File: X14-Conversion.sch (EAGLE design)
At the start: 23 parts, among them P1 282837-2, P2 282837-2, P3 282837-2

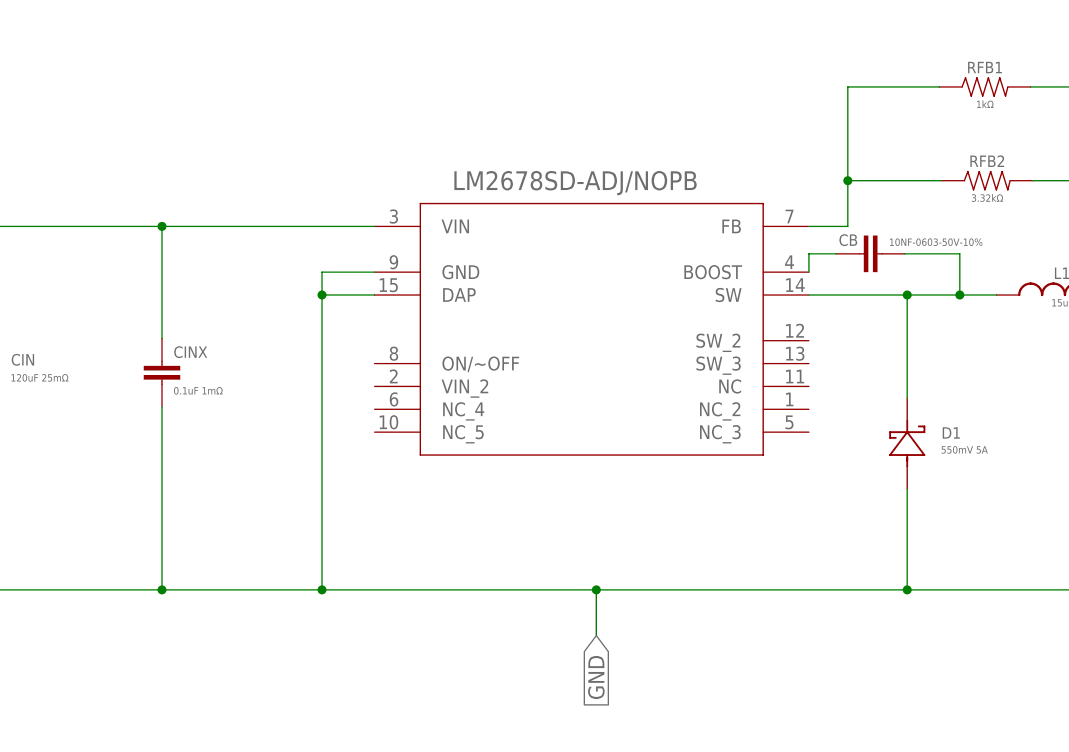
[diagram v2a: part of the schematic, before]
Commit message: Fix Board Layout
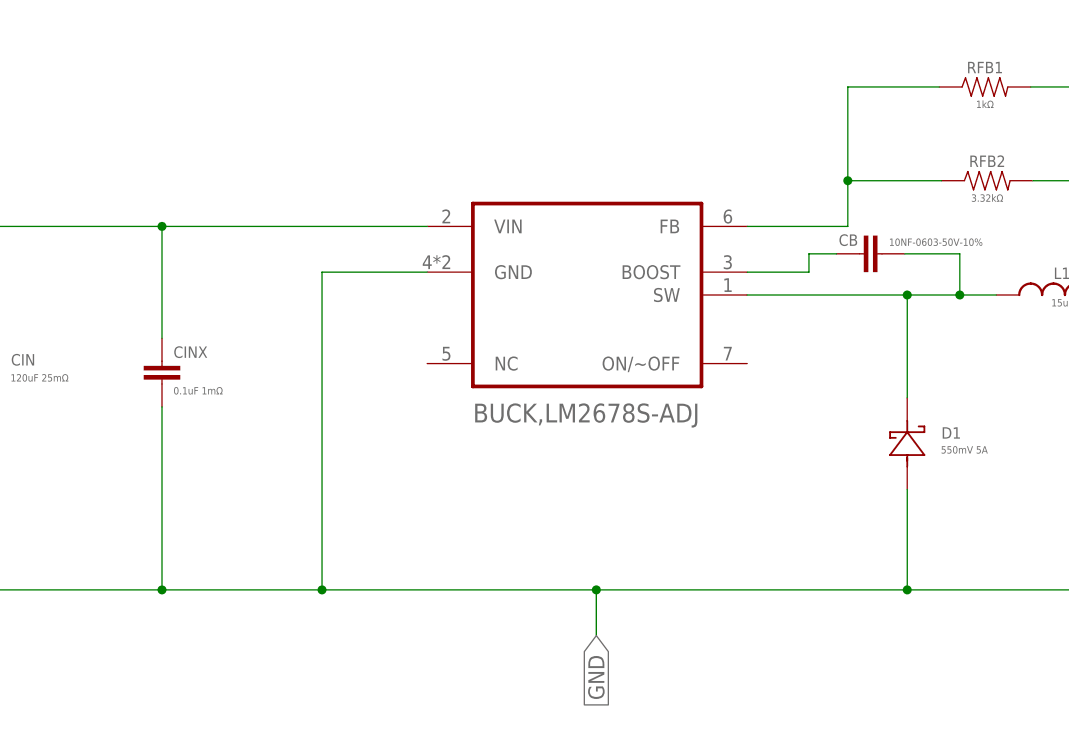
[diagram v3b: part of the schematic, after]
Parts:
- removed LM2678: LM2678SD-ADJ/NOPB, LM2678SX-ADJNOPB:LM2678SD-ADJ/NOPB
- added U1: BUCK,LM2678S-ADJ, BUCK, LM2678S-ADJ:BUCK,LM2678S-ADJ
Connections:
- net 12V: now also U1.VIN; no longer LM2678.VIN
- net GND: now also U1.GND; no longer LM2678.DAP, LM2678.GND
- net N$2: now also U1.SW; no longer LM2678.SW
- net N$4: now also U1.BOOST; no longer LM2678.BOOST
- net N$5: now also U1.FB; no longer LM2678.FB
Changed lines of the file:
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@@
 <part name="FRAME1" library="frames" library_urn="urn:adsk.eagle:library:229" deviceset="A3L-LOC" device=""/>
 <part name="AZ1117C" library="AZ1117C-3.3" deviceset="SOT150P410X160-3N" device="" value="AZ1117C-3.3"/>
-<part name="LM2678" library="LM2678SX-ADJNOPB" deviceset="LM2678SD-ADJ/NOPB" device=""/>
 <part name="U$2" library="testpoints" deviceset="3.3V_TESTPOINT" device=""/>
 <part name="U$3" library="testpoints" deviceset="5.2V_TESTPOINT" device=""/>
@@
 <part name="C3" library="SparkFun-Capacitors" library_urn="urn:adsk.eagle:library:510" deviceset="0.1UF" device="-0603-25V-(+80/-20%)" package3d_urn="urn:adsk.eagle:package:37414/1" value="0.1uF"/>
 <part name="CONN" library="CONN, Distribution-Conversion (3)" deviceset="CONVERSION-DISTRIBUTION" device=""/>
+<part name="U1" library="BUCK, LM2678S-ADJ" deviceset="BUCK,LM2678S-ADJ" device=""/>
 </parts>
 <sheets>
@@
 </instance>
 <instance part="AZ1117C" gate="G$1" x="-75.692" y="-10.668" smashed="yes"/>
-<instance part="LM2678" gate="A" x="-2.54" y="66.04" smashed="yes">
-<attribute name="NAME" x="-13.6144" y="79.9846" size="2.0828" layer="95" ratio="6" rot="SR0" display="off"/>
-<attribute name="VALUE" x="-13.4874" y="77.4446" size="2.0828" layer="96" ratio="6" rot="SR0"/>
-</instance>
 <instance part="U$2" gate="G$1" x="17.78" y="-2.54" smashed="yes"/>
 <instance part="U$3" gate="G$1" x="17.78" y="-12.7" smashed="yes"/>
@@
 <instance part="CONN" gate="G$1" x="-81.28" y="-81.28" smashed="yes">
 <attribute name="NAME" x="-88.9" y="-73.66" size="1.778" layer="95"/>
+</instance>
+<instance part="U1" gate="A" x="1.524" y="65.786" smashed="yes">
+<attribute name="NAME" x="-11.176" y="76.946" size="2.0828" layer="95" ratio="10" rot="SR0" display="off"/>
+<attribute name="VALUE" x="-11.176" y="51.626" size="2.0828" layer="96" ratio="10" rot="SR0"/>
 </instance>
 </instances>
@@
 <wire x1="-45.72" y1="33.02" x2="-27.94" y2="33.02" width="0.1524" layer="91"/>
 <junction x="2.54" y="33.02"/>
-<pinref part="LM2678" gate="A" pin="GND"/>
 <wire x1="-27.94" y1="33.02" x2="2.54" y2="33.02" width="0.1524" layer="91"/>
-<wire x1="-22.098" y1="68.326" x2="-27.94" y2="68.326" width="0.1524" layer="91"/>
-<wire x1="-27.94" y1="68.326" x2="-27.94" y2="65.786" width="0.1524" layer="91"/>
 <junction x="-27.94" y="33.02"/>
-<pinref part="LM2678" gate="A" pin="DAP"/>
-<wire x1="-27.94" y1="65.786" x2="-27.94" y2="33.02" width="0.1524" layer="91"/>
-<wire x1="-22.098" y1="65.786" x2="-27.94" y2="65.786" width="0.1524" layer="91"/>
-<junction x="-27.94" y="65.786"/>
+<wire x1="-27.94" y1="68.326" x2="-27.94" y2="33.02" width="0.1524" layer="91"/>
 <wire x1="-45.72" y1="33.02" x2="-66.04" y2="33.02" width="0.1524" layer="91"/>
 <wire x1="-66.04" y1="33.02" x2="-66.04" y2="53.34" width="0.1524" layer="91"/>
@@
 <pinref part="CIN" gate="G$1" pin="2"/>
 <pinref part="C3" gate="G$1" pin="2"/>
+<pinref part="U1" gate="A" pin="GND"/>
+<wire x1="-27.94" y1="68.326" x2="-16.256" y2="68.326" width="0.1524" layer="91"/>
 </segment>
 <segment>
@@
 <net name="12V" class="0">
 <segment>
-<pinref part="LM2678" gate="A" pin="VIN"/>
-<wire x1="-22.098" y1="73.406" x2="-45.72" y2="73.406" width="0.1524" layer="91"/>
+<wire x1="-16.256" y1="73.406" x2="-45.72" y2="73.406" width="0.1524" layer="91"/>
 <wire x1="-45.72" y1="73.406" x2="-45.72" y2="60.96" width="0.1524" layer="91"/>
 <wire x1="-66.04" y1="60.96" x2="-66.04" y2="73.406" width="0.1524" layer="91"/>
@@
 <pinref part="CINX" gate="G$1" pin="1"/>
 <pinref part="CIN" gate="G$1" pin="1"/>
+<pinref part="U1" gate="A" pin="VIN"/>
 </segment>
 <segment>
@@
 <net name="N$2" class="0">
 <segment>
-<pinref part="LM2678" gate="A" pin="SW"/>
 <pinref part="L1" gate="G$1" pin="1"/>
-<wire x1="26.162" y1="65.786" x2="37.084" y2="65.786" width="0.1524" layer="91"/>
+<wire x1="19.304" y1="65.786" x2="37.084" y2="65.786" width="0.1524" layer="91"/>
 <wire x1="37.084" y1="65.786" x2="42.926" y2="65.786" width="0.1524" layer="91"/>
 <wire x1="42.926" y1="65.786" x2="46.99" y2="65.786" width="0.1524" layer="91"/>
@@
 <pinref part="CB" gate="G$1" pin="2"/>
 <pinref part="D1" gate="A" pin="1"/>
+<pinref part="U1" gate="A" pin="SW"/>
 </segment>
 </net>
 <net name="N$4" class="0">
 <segment>
-<pinref part="LM2678" gate="A" pin="BOOST"/>
 <wire x1="26.162" y1="68.326" x2="26.162" y2="70.358" width="0.1524" layer="91"/>
 <wire x1="26.162" y1="70.358" x2="29.21" y2="70.358" width="0.1524" layer="91"/>
 <pinref part="CB" gate="G$1" pin="1"/>
+<pinref part="U1" gate="A" pin="BOOST"/>
+<wire x1="26.162" y1="68.326" x2="19.304" y2="68.326" width="0.1524" layer="91"/>
 </segment>
 </net>
 <net name="N$5" class="0">
 <segment>
-<pinref part="LM2678" gate="A" pin="FB"/>
-<wire x1="26.162" y1="73.406" x2="30.48" y2="73.406" width="0.1524" layer="91"/>
 <wire x1="30.48" y1="73.406" x2="30.48" y2="78.486" width="0.1524" layer="91"/>
 <wire x1="30.48" y1="78.486" x2="40.894" y2="78.486" width="0.1524" layer="91"/>
@@
 <pinref part="RFB1" gate="G$1" pin="1"/>
 <pinref part="RFB2" gate="G$1" pin="1"/>
-</segment>
-</net>
+<pinref part="U1" gate="A" pin="FB"/>
+<wire x1="30.48" y1="73.406" x2="19.304" y2="73.406" width="0.1524" layer="91"/>
+</segment>
+</net>
